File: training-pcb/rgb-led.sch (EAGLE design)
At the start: 19 parts, among them J1 MICRO-USB, J2 AVR_SPI_PROG2PTH2, U1 ATTINY441/841SSU/SSUR, U2 TCA6507PW, U3 TLV70018DDCR

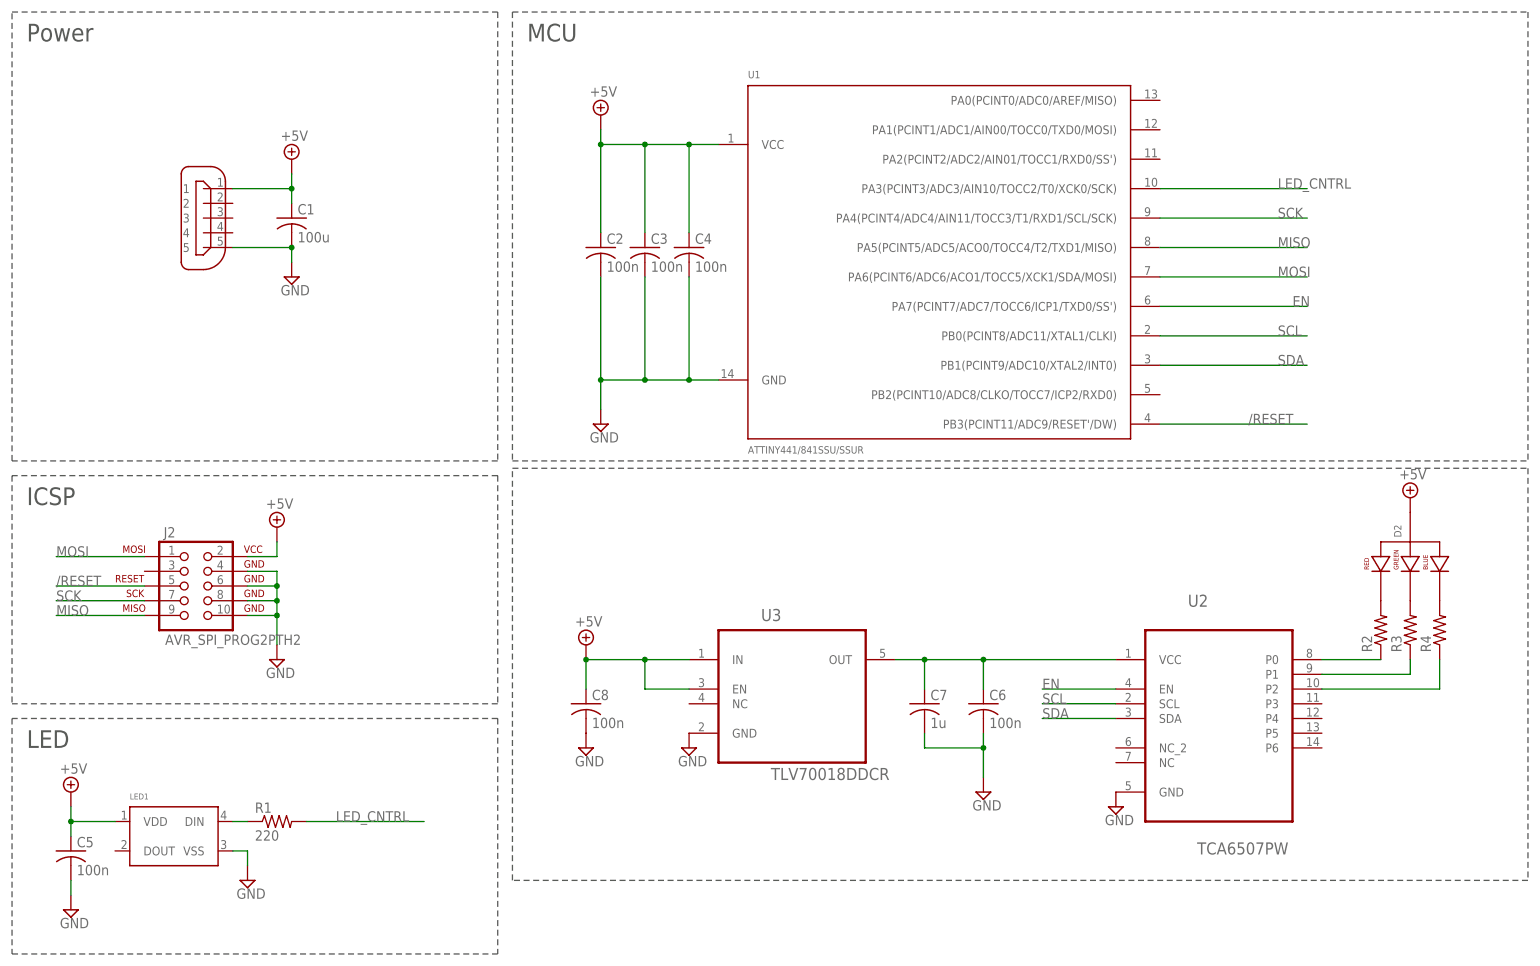
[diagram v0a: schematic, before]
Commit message: Switched RGB LED driver ICs, added button, NEEDS ROUTING
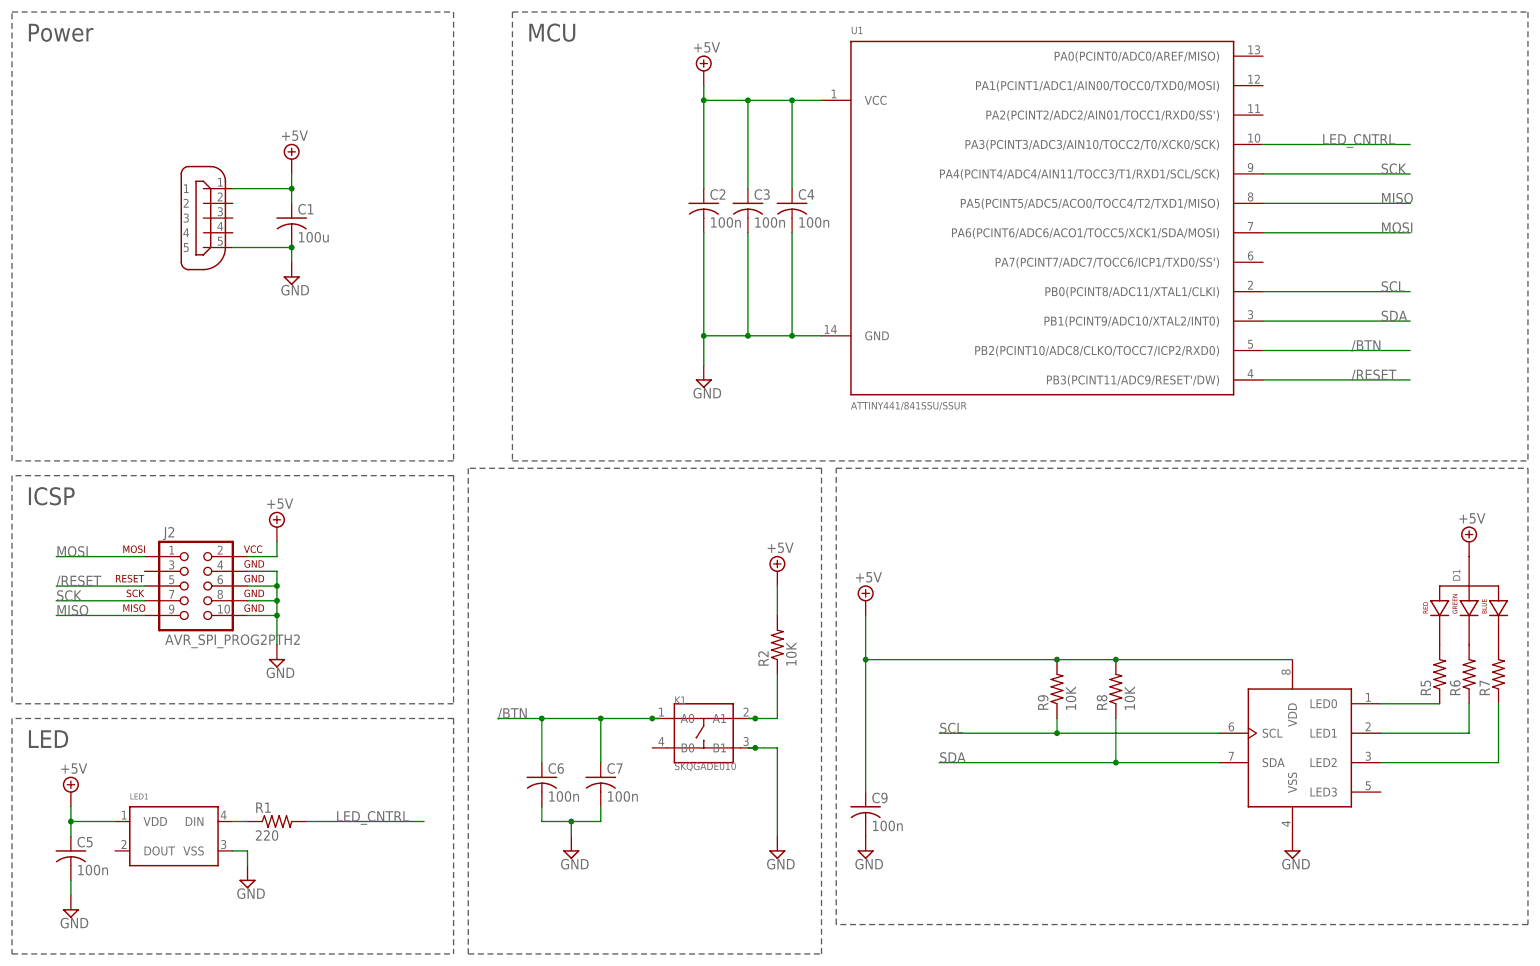
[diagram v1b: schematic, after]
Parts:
- removed C8: 100n, rcl:C-USC0603
- removed D2: LED-RGB-CA-THRUCLEAR, rgb-led:LED-RGB-CA-THRUCLEAR
- removed R3, R4: (no value), resistor:R-US_R0805
- removed U2: TCA6507PW, rgb-led:TCA6507PW
- removed U3: TLV70018DDCR, rgb-led:TLV70018DDCR
- added C9: 100n, rcl:C-USC0603
- added D1: LED-RGB-CA-THRUCLEAR, rgb-led:LED-RGB-CA-THRUCLEAR
- added K1: SKQGADE010, Seeed-OPL-Button:SMD-SWITCH-TOP-260GF(4P-D5.2MM)
- added R5, R6, R7: (no value), resistor:R-US_R0805
- added R8, R9: 10K, resistor:R-US_R0805
- added U$1: PCA9533, adam - ics:PCA9533
- C7: value 1u -> 100n
- R2: value (none) -> 10K
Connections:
- removed net +1.8V: C6.1, C7.1, U2.VCC, U3.OUT
- removed net EN: U1.PA7(PCINT7/ADC7/TOCC6/ICP1/TXD0/SS'), U2.EN
- removed net N$3: R2.1, U2.P0
- removed net N$4: R3.1, U2.P1
- removed net N$5: R4.1, U2.P2
- removed net N$7: D2.GREEN_CATHODE, R3.2
- removed net N$8: D2.BLUE_CATHODE, R4.2
- new net /BTN: C6.1, C7.1, K1.A0, U1.PB2(PCINT10/ADC8/CLKO/TOCC7/ICP2/RXD0)
- new net N$10: D1.BLUE_CATHODE, R7.2
- new net N$11: R5.1, U$1.LED0
- new net N$12: R6.1, U$1.LED1
- new net N$13: R7.1, U$1.LED2
- new net N$6: D1.RED_CATHODE, R5.2
- new net N$9: D1.GREEN_CATHODE, R6.2
- net +5V: now also C9.1, D1.ANODE, R2.2, R8.2, R9.2, U$1.VDD; no longer C8.1, D2.ANODE, U3.EN, U3.IN
- net GND: now also C9.2, K1.B1, U$1.VSS; no longer C8.2, U2.GND, U3.GND
- net N$2: now also K1.A1, R2.1; no longer D2.RED_CATHODE, R2.2
- net SCL: now also R9.1, U$1.SCL; no longer U2.SCL
- net SDA: now also R8.1, U$1.SDA; no longer U2.SDA
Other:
- moved on the sheet: C2, C3, C4, C6, C7, R2, U1
